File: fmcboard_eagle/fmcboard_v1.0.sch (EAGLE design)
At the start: 14 parts, among them IC1 OPA699ID, IC2 OPA699ID, J1 8pin, J12 4p-2.54, J2 ASP-134604-01, J3 4p-2.54, J4 4p-2.54

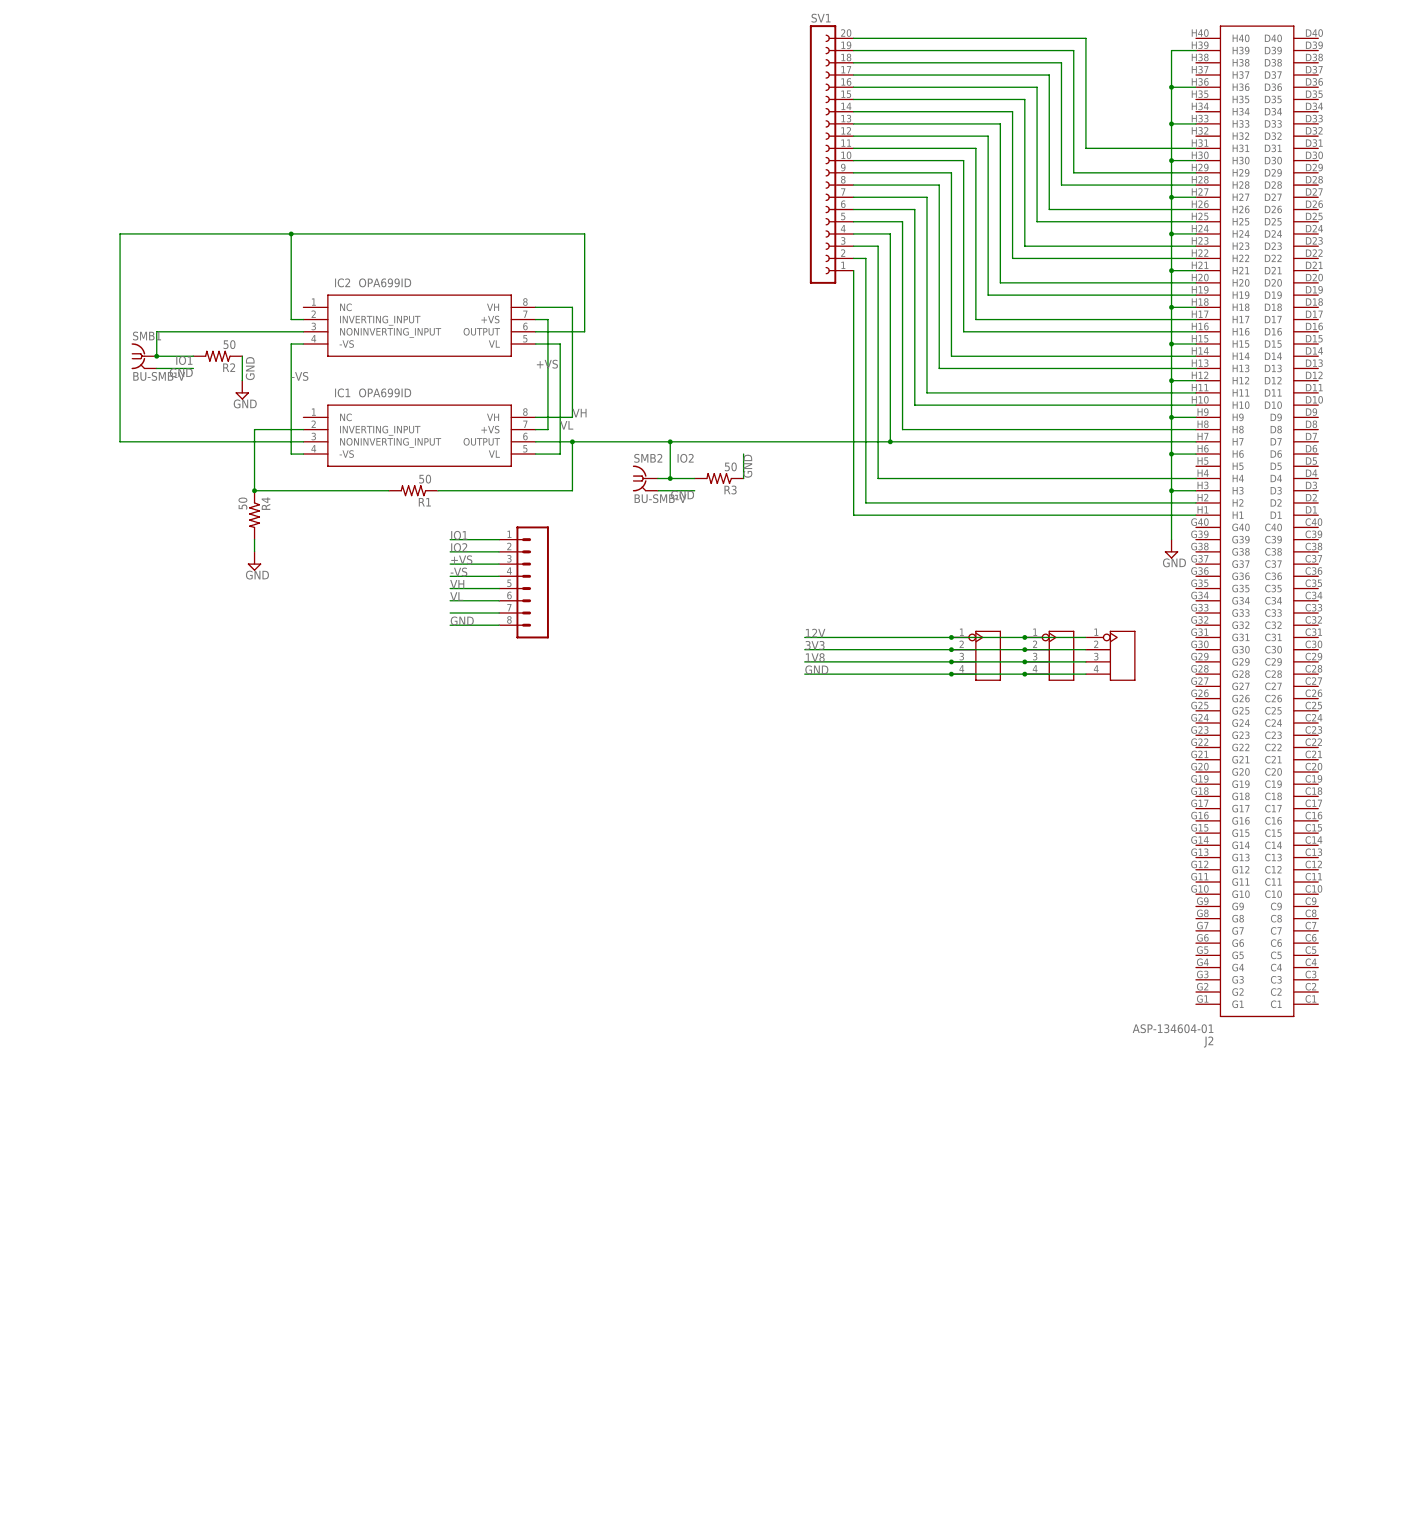
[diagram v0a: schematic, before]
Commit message: board v1 work with Andre
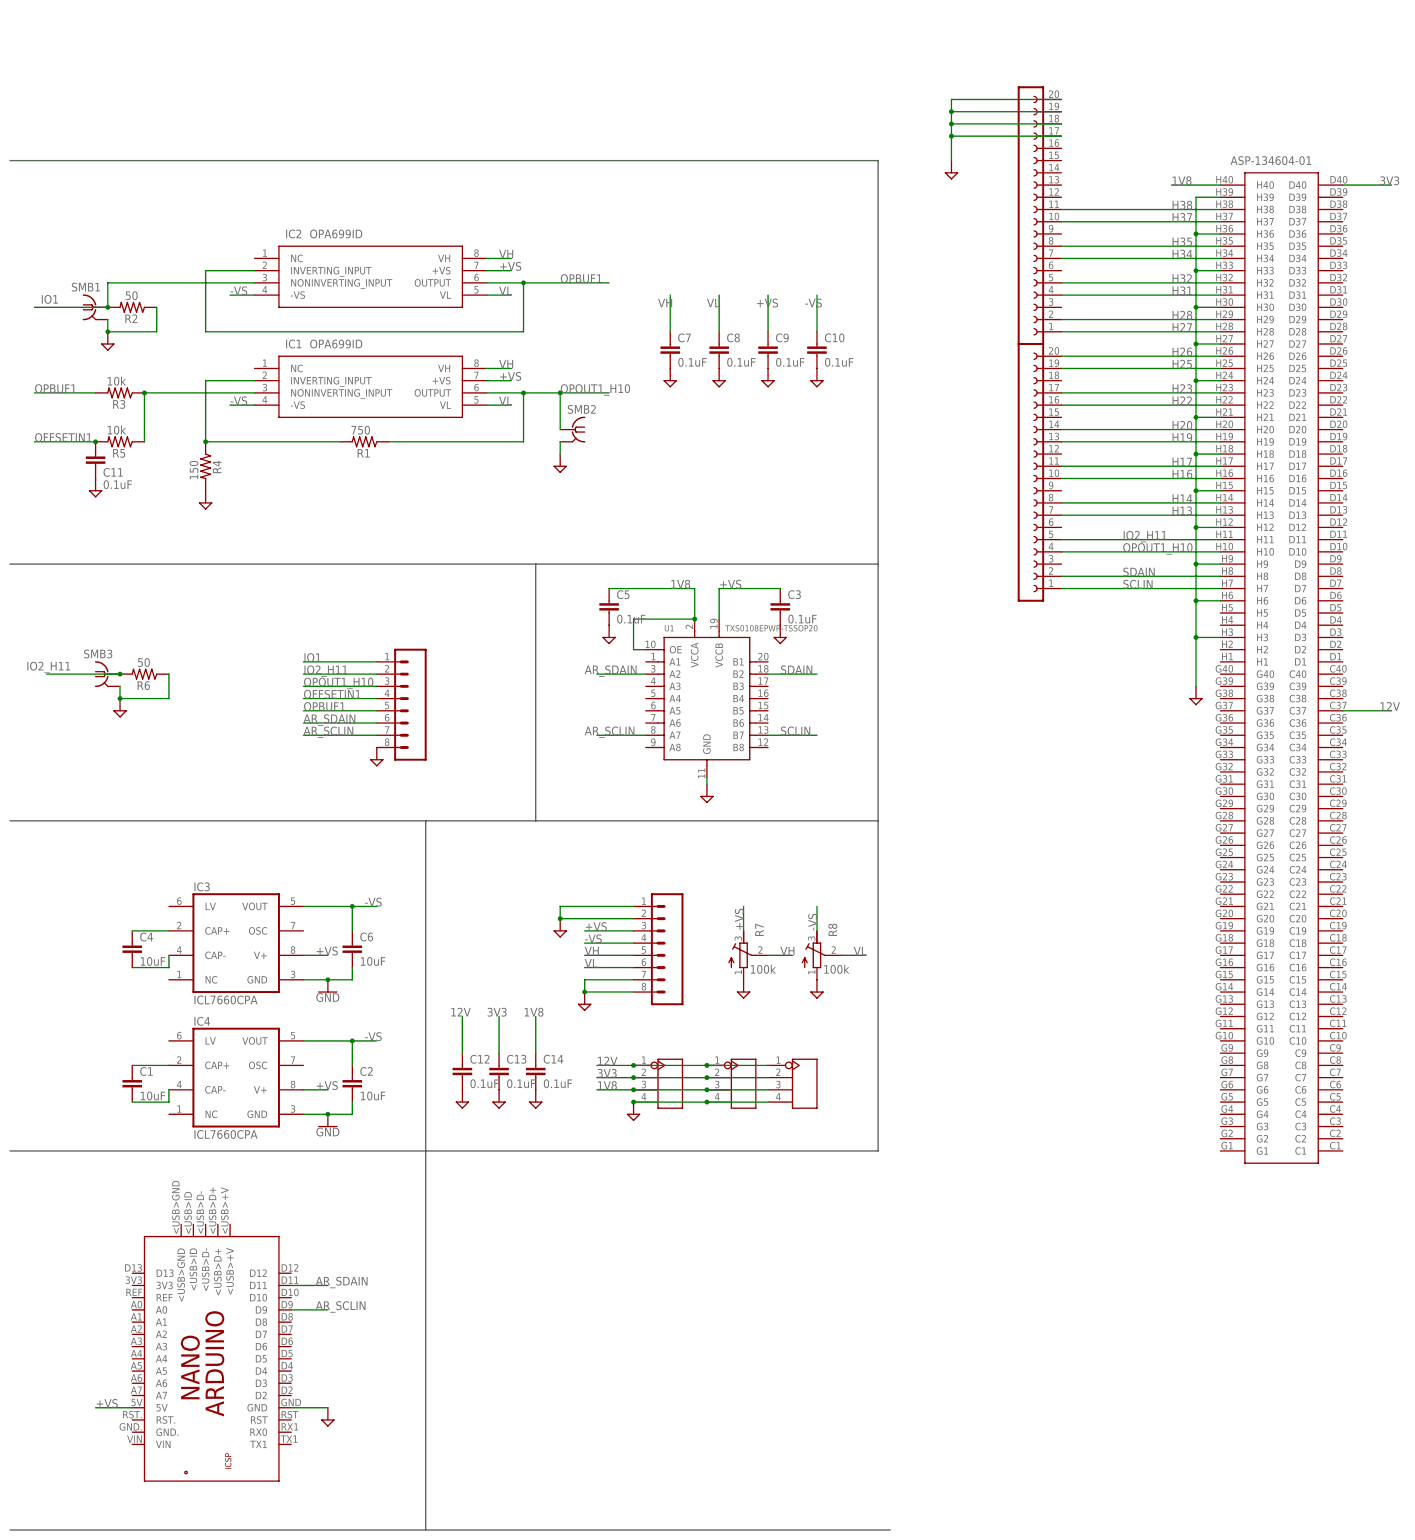
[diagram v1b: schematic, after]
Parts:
- added C1, C2, C4, C6: 10uF, SparkFun-Capacitors:CAPPTH1
- added C10, C11, C12, C13, C14, C3, C5, C7, C8, C9: 0.1uF, SparkFun-Passives:CAP0805
- added IC3, IC4: ICL7660CPA, maxim:ICL7660CPA
- added J5: 8pin, SparkFun-Connectors:CONN_08"
- added PCB1: ARDUINO_NANO, E14_Arduino_revC:ARDUINO_NANO
- added R5: 10k, SparkFun-Resistors:RESISTORAXIAL-0.3
- added R6: 50, SparkFun-Resistors:RESISTORAXIAL-0.3
- added R7, R8: 100k, resistor:R-TRIMM3296W
- added SMB3: BU-SMB-V, con-coax:BU-SMB-V
- added SV2: 20, con-lsta:FE20-1
- added U1: TXS0108EPWR-TSSOP20, Seeed-IC:LOGIC-TXS0108EPWR(TSSOP20)
- R1: value 50 -> 750
- R3: value 50 -> 10k
- R4: value 50 -> 150
- SV1: value (none) -> 20
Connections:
- net N$16 renamed H16
- net N$17 renamed H17
- removed net IO2: IC1.OUTPUT, J1.2, J2.H7, R1.1, R3.2, SMB2.1, SV1.4
- removed net N$10: J2.H8, SV1.5
- removed net N$11: J2.H4, SV1.3
- removed net N$12: J2.H10, SV1.6
- removed net N$13: J2.H11, SV1.7
- removed net N$14: J2.H13, SV1.8
- removed net N$15: J2.H14, SV1.9
- removed net N$18: J2.H19, SV1.12
- removed net N$19: J2.H20, SV1.13
- removed net N$20: J2.H22, SV1.14
- removed net N$21: J2.H23, SV1.15
- removed net N$22: J2.H25, SV1.16
- removed net N$23: J2.H26, SV1.17
- removed net N$24: J2.H28, SV1.18
- removed net N$25: J2.H29, SV1.19
- removed net N$26: J2.H31, SV1.20
- removed net N$7: J1.7
- removed net N$8: J2.H1, SV1.1
- removed net N$9: J2.H2, SV1.2
- new net AR_SCLIN: J5.7, PCB1.D9, U1.A7
- new net AR_SDAIN: J5.6, PCB1.D11, U1.A2
- new net H13: J2.H13, SV1.7
- new net H14: J2.H14, SV1.8
- new net H19: J2.H19, SV1.13
- new net H20: J2.H20, SV1.14
- new net H22: J2.H22, SV1.16
- new net H23: J2.H23, SV1.17
- new net H25: J2.H25, SV1.19
- new net H26: J2.H26, SV1.20
- new net H27: J2.H28, SV2.1
- new net H28: J2.H29, SV2.2
- new net H31: J2.H31, SV2.4
- new net H32: J2.H32, SV2.5
- new net H34: J2.H34, SV2.7
- new net H35: J2.H35, SV2.8
- new net H37: J2.H37, SV2.10
- new net H38: J2.H38, SV2.11
- new net IO2_H11: J2.H11, J5.2, R6.2, SMB3.1, SV1.5
- new net N$2: C4.1, IC3.CAP+
- new net N$4: C4.2, IC3.CAP-
- new net N$5: C1.1, IC4.CAP+
- new net N$6: C1.2, IC4.CAP-
- new net OFFSETIN1: C11.1, J5.4, R5.2
- new net OPBUF1: IC2.INVERTING_INPUT, IC2.OUTPUT, J5.5, R3.2
- new net OPOUT1_H10: IC1.OUTPUT, J2.H10, J5.3, R1.1, SMB2.1, SV1.4
- new net SCLIN: J2.H7, SV1.1, U1.B7
- new net SDAIN: J2.H8, SV1.2, U1.B2
- net +VS: now also C3.1, C9.1, IC3.V+, IC4.V+, PCB1.5V, R7.E, U1.VCCB
- net -VS: now also C10.1, C2.1, C6.1, IC3.VOUT, IC4.VOUT, R8.E
- net 12V: now also C12.1, J2.C37
- net 1V8: now also C14.1, C5.1, J2.H40, U1.OE, U1.VCCA
- net 3V3: now also C13.1, J2.D40
- net GND: now also C10.2, C11.2, C12.2, C13.2, C14.2, C2.2, C3.2, C5.2, C6.2, C7.2, C8.2, C9.2, IC3.GND, IC4.GND, J1.1, J1.2, J1.7, J5.8, PCB1.GND, R6.1, R7.A, R8.A, SMB3.2, SV2.17, SV2.18, SV2.19, SV2.20, U1.GND; no longer R3.1
- net IO1: now also J5.1; no longer J1.1
- net N$1: now also R3.1, R5.1; no longer IC2.INVERTING_INPUT, IC2.OUTPUT
- net VH: now also C7.1, R7.S
- net VL: now also C8.1, R8.S
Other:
- note added: "FMC breakout"
- note added: "IO"
- note added: "Level shifter"
- note added: "Negative V supply"
- note added: "Op amps"
- note added: "Power inputs"
- moved on the sheet: IC1, IC2, R1, R2, R3, R4, SMB1, SMB2

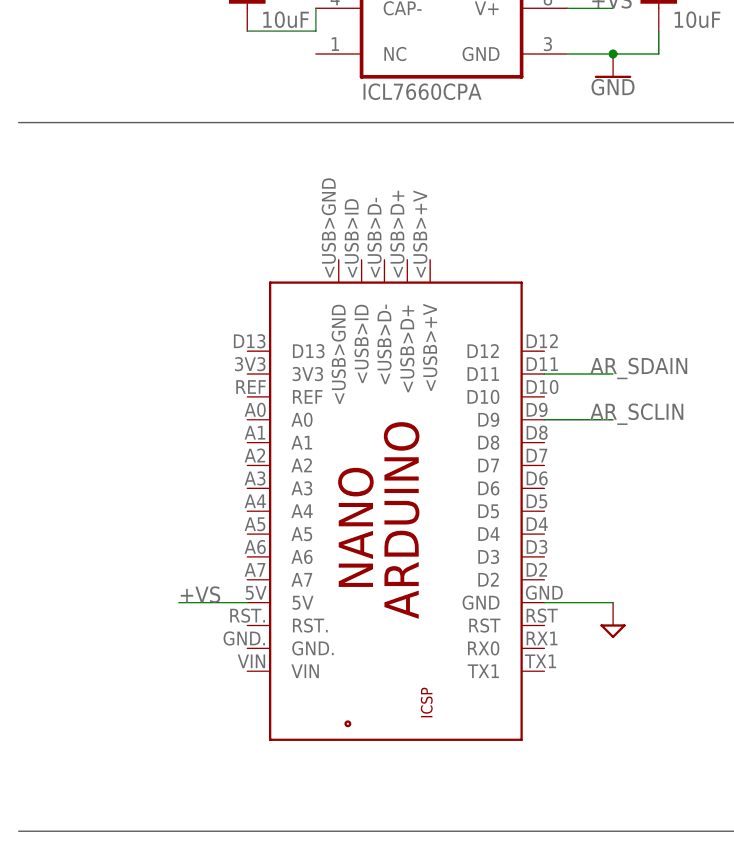
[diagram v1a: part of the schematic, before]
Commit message: first draft of pcb routing
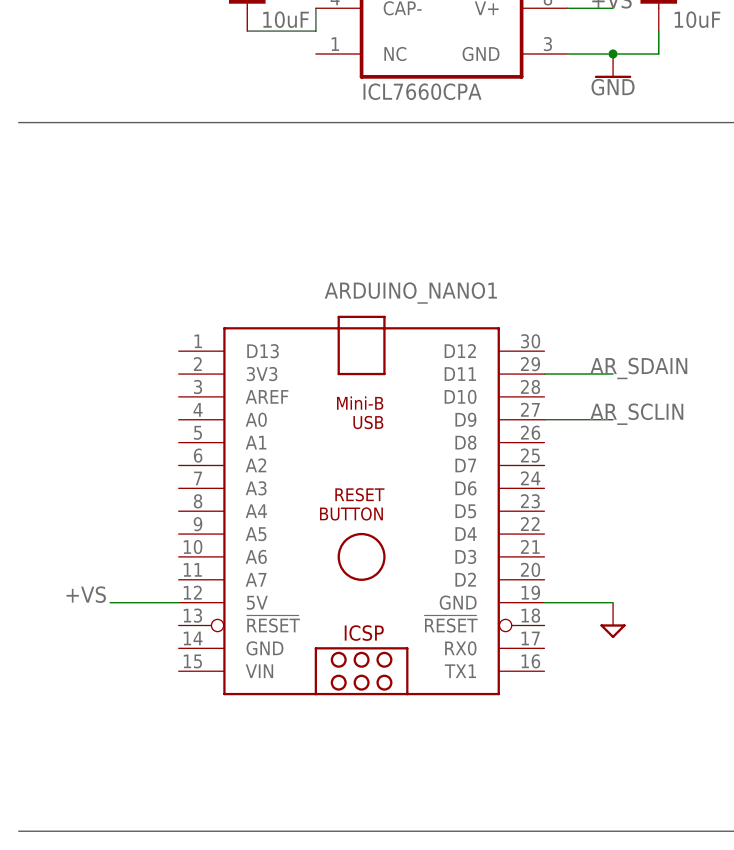
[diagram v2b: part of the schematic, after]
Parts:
- removed PCB1: ARDUINO_NANO, E14_Arduino_revC:ARDUINO_NANO
- added ARDUINO_NANO1: (no value), ArduinoNanoV30:ARDUINO_NANO
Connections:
- net +VS: now also ARDUINO_NANO1.5V; no longer PCB1.5V
- net AR_SCLIN: now also ARDUINO_NANO1.D9; no longer PCB1.D9
- net AR_SDAIN: now also ARDUINO_NANO1.D11; no longer PCB1.D11
- net GND: now also ARDUINO_NANO1.GND@1; no longer PCB1.GND
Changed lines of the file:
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@@
 <part name="SUPPLY22" library="supply2" library_urn="urn:adsk.eagle:library:372" deviceset="GND" device=""/>
 <part name="SUPPLY23" library="supply2" library_urn="urn:adsk.eagle:library:372" deviceset="GND" device=""/>
-<part name="PCB1" library="E14_Arduino_revC" deviceset="ARDUINO_NANO" device=""/>
 <part name="SUPPLY24" library="supply2" library_urn="urn:adsk.eagle:library:372" deviceset="GND" device=""/>
+<part name="ARDUINO_NANO1" library="ArduinoNanoV30" deviceset="ARDUINO_NANO" device=""/>
 </parts>
 <sheets>
@@
 <instance part="SUPPLY22" gate="GND" x="154.94" y="20.32" smashed="yes"/>
 <instance part="SUPPLY23" gate="GND" x="170.18" y="20.32" smashed="yes"/>
-<instance part="PCB1" gate="G$1" x="45.72" y="-55.88" smashed="yes" rot="R270"/>
 <instance part="SUPPLY24" gate="GND" x="68.58" y="-68.58" smashed="yes"/>
+<instance part="ARDUINO_NANO1" gate="G$1" x="40.64" y="-60.96" smashed="yes" rot="R180">
+<attribute name="NAME" x="55.88" y="-30.48" size="1.778" layer="95" rot="R180"/>
+<attribute name="VALUE" x="55.88" y="-27.94" size="1.778" layer="96" rot="R180"/>
+</instance>
 </instances>
 <busses>
@@
 </segment>
 <segment>
-<pinref part="PCB1" gate="G$1" pin="GND"/>
 <wire x1="60.96" y1="-66.04" x2="68.58" y2="-66.04" width="0.1524" layer="91"/>
 <pinref part="SUPPLY24" gate="GND" pin="GND"/>
+<pinref part="ARDUINO_NANO1" gate="G$1" pin="GND@1"/>
 </segment>
 </net>
@@
 </segment>
 <segment>
-<pinref part="PCB1" gate="G$1" pin="5V"/>
-<wire x1="27.94" y1="-66.04" x2="20.32" y2="-66.04" width="0.1524" layer="91"/>
-<label x="20.32" y="-66.04" size="1.778" layer="95"/>
+<wire x1="20.32" y1="-66.04" x2="12.7" y2="-66.04" width="0.1524" layer="91"/>
+<label x="7.62" y="-66.04" size="1.778" layer="95"/>
+<pinref part="ARDUINO_NANO1" gate="G$1" pin="5V"/>
 </segment>
 </net>
@@
 </segment>
 <segment>
-<pinref part="PCB1" gate="G$1" pin="D11"/>
 <wire x1="60.96" y1="-40.64" x2="68.58" y2="-40.64" width="0.1524" layer="91"/>
 <label x="66.04" y="-40.64" size="1.778" layer="95"/>
+<pinref part="ARDUINO_NANO1" gate="G$1" pin="D11"/>
 </segment>
 </net>
@@
 </segment>
 <segment>
-<pinref part="PCB1" gate="G$1" pin="D9"/>
 <wire x1="60.96" y1="-45.72" x2="68.58" y2="-45.72" width="0.1524" layer="91"/>
 <label x="66.04" y="-45.72" size="1.778" layer="95"/>
+<pinref part="ARDUINO_NANO1" gate="G$1" pin="D9"/>
 </segment>
 </net>
@@
 </drawing>
 <compatibility>
+<note version="6.3" minversion="6.2.2" severity="warning">
+Since Version 6.2.2 text objects can contain more than one line,
+which will not be processed correctly with this version.
+</note>
 <note version="8.2" severity="warning">
 Since Version 8.2, EAGLE supports online libraries. The ids
